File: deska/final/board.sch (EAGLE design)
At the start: 86 parts, among them IC1 DSPIC33EP256MU806-X_PT, IC2 TP4056, SW1 KSS-2EG4430, SW2 KSS-2EG4430, SW3 KSS-2EG4430, U1 TPS731, X1 MINI-USB-UX60-MB-5ST

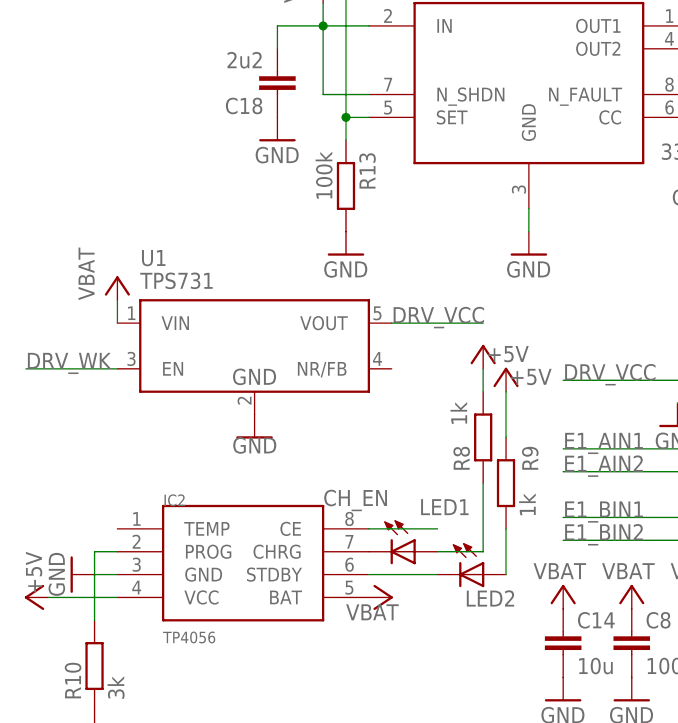
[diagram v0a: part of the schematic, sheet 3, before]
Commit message: psani HW
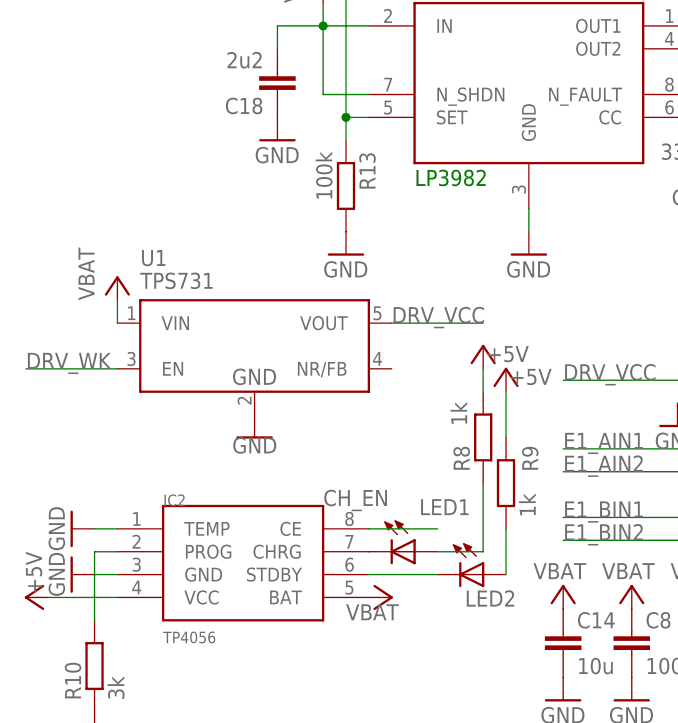
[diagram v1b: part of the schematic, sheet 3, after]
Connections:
- net GND: now also IC2.TEMP
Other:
- note added: "LP3982"
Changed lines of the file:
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@@
 <part name="GND28" library="SparkFun-Aesthetics" deviceset="GND" device=""/>
 <part name="GND29" library="SparkFun-Aesthetics" deviceset="GND" device=""/>
+<part name="GND30" library="SparkFun-Aesthetics" deviceset="GND" device=""/>
 </parts>
 <sheets>
@@
 <sheet>
 <plain>
+<text x="-2.54" y="96.52" size="1.778" layer="91">LP3982</text>
 </plain>
 <instances>
@@
 </instance>
 <instance part="U$46" gate="G$1" x="-35.56" y="83.82"/>
+<instance part="GND30" gate="1" x="-40.64" y="58.42" rot="R270"/>
 </instances>
 <busses>
@@
 <pinref part="GND87" gate="1" pin="GND"/>
 </segment>
-</net>
+<segment>
+<pinref part="IC2" gate="G$1" pin="TEMP"/>
+<pinref part="GND30" gate="1" pin="GND"/>
+<wire x1="-35.56" y1="58.42" x2="-38.1" y2="58.42" width="0.1524" layer="91"/>
+</segment>
+</net>
